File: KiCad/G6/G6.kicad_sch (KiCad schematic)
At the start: 7 parts, among them J2 Conn_02x20_Odd_Even_MountingP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, Q1 2N3904, U11 SN74HC74DRG4 (SOIC14)

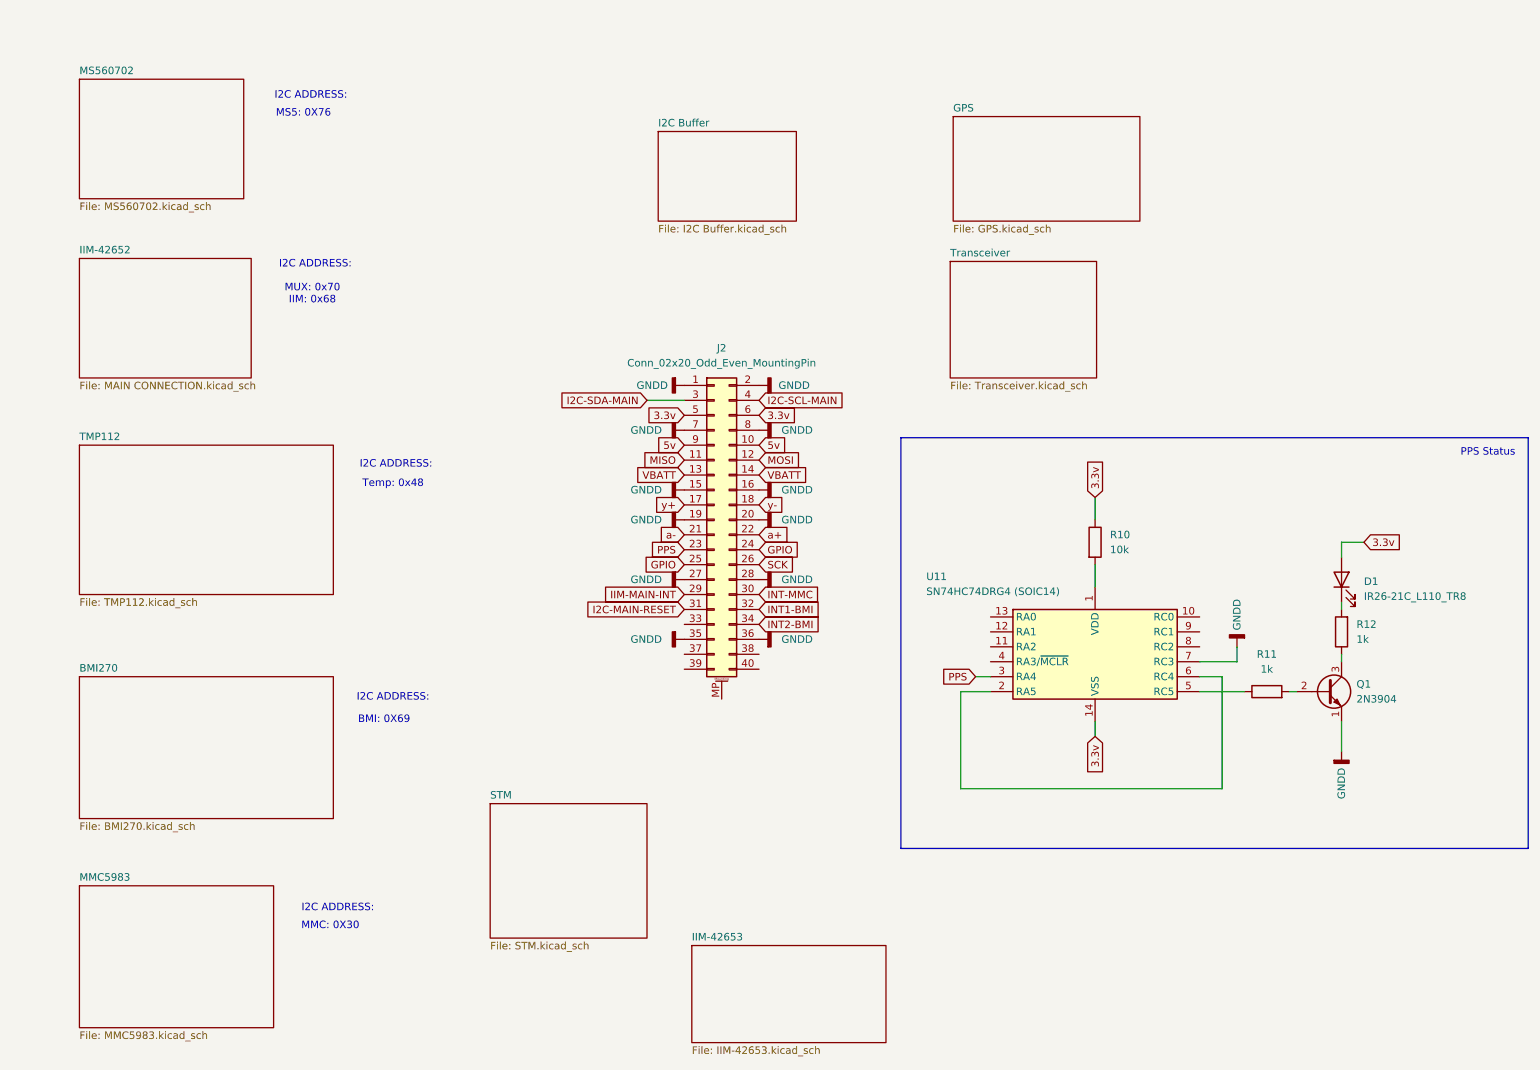
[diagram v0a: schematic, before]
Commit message: I think the schematics done uhhh idrk
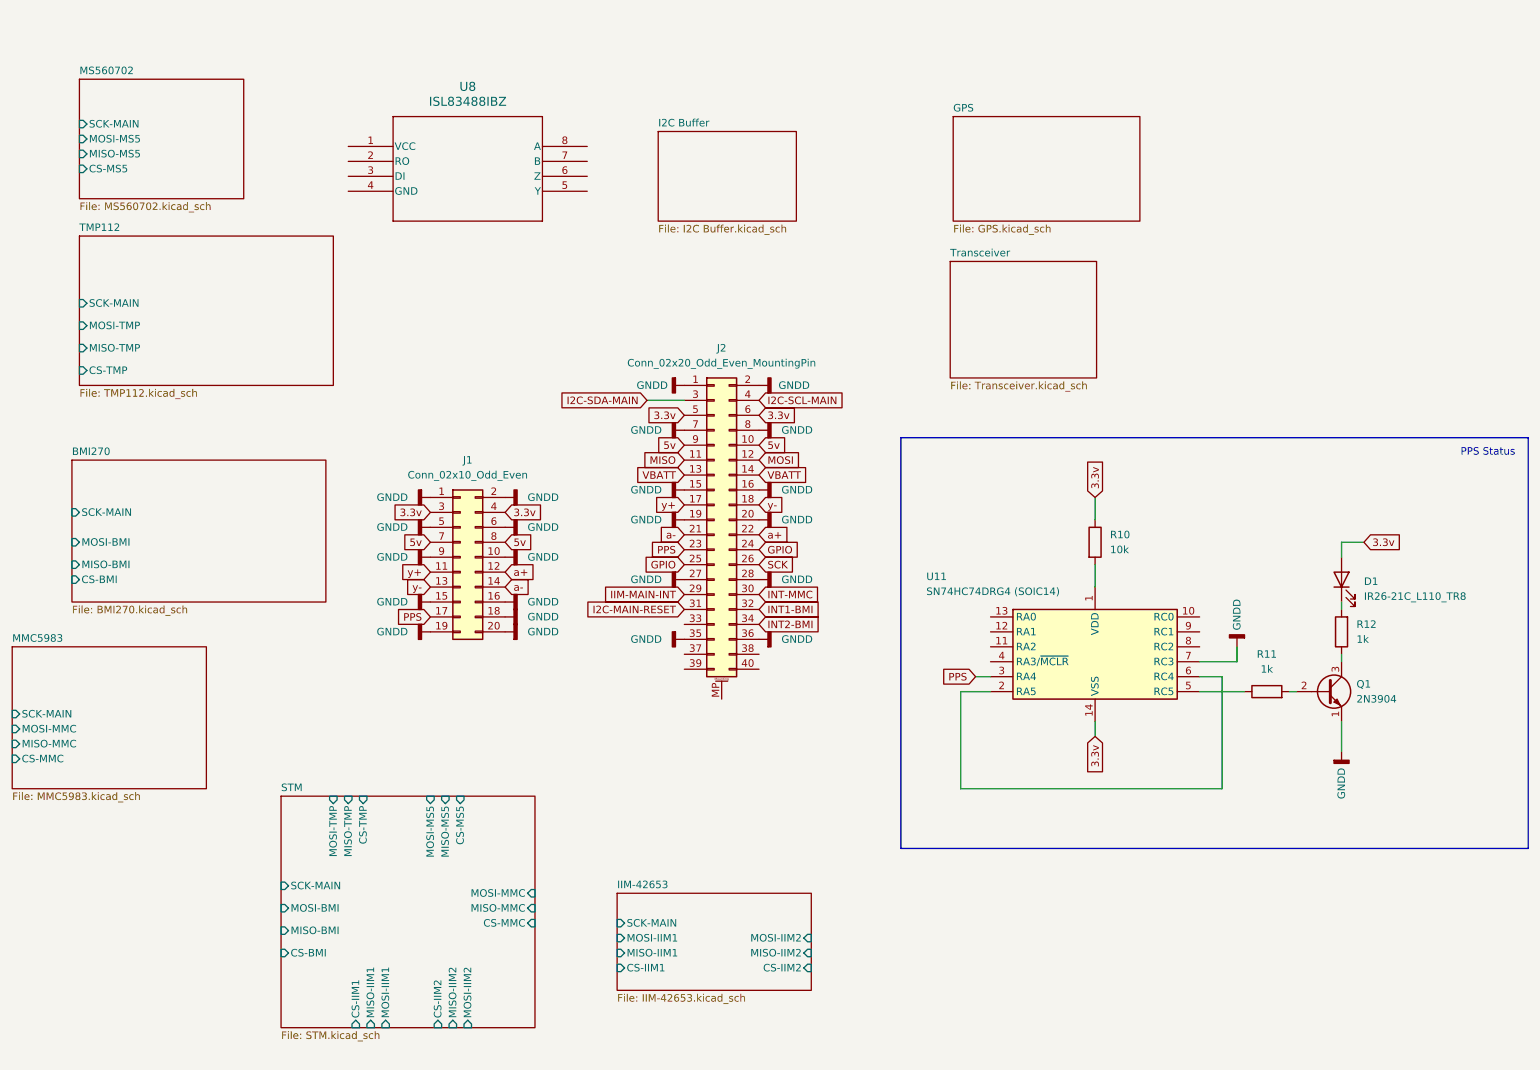
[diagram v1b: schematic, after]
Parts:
- added J1: Conn_02x10_Odd_Even, Connector_PinHeader_2.54mm:PinHeader_2x10_P2.54mm_Vertical, symbol Connector_Generic:Conn_02x10_Odd_Even
- added U8: ISL83488IBZ, CC0603KRXQRQBB104:SOIC8_4X5_INR, symbol ISL83488IBZ:ISL83488IBZ
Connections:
- net 3.3v: now also J1.3 (Pin_3), J1.4 (Pin_4)
- net 5v: now also J1.7 (Pin_7), J1.8 (Pin_8)
- net GNDD: now also J1.1 (Pin_1), J1.10 (Pin_10), J1.15 (Pin_15), J1.16 (Pin_16), J1.18 (Pin_18), J1.19 (Pin_19), J1.2 (Pin_2), J1.20 (Pin_20), J1.5 (Pin_5), J1.6 (Pin_6), J1.9 (Pin_9)
- net PPS: now also J1.17 (Pin_17)
- net a+: now also J1.12 (Pin_12)
- net a-: now also J1.14 (Pin_14)
- net y+: now also J1.11 (Pin_11)
- net y-: now also J1.13 (Pin_13)
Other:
- removed sheet IIM-42652
- sheet BMI270 ports: added CS-BMI, MISO-BMI, MOSI-BMI, SCK-MAIN; removed none
- sheet IIM-42653 ports: added CS-IIM1, CS-IIM2, MISO-IIM1, MISO-IIM2, MOSI-IIM1, MOSI-IIM2, SCK-MAIN; removed none
- sheet MMC5983 ports: added CS-MMC, MISO-MMC, MOSI-MMC, SCK-MAIN; removed none
- sheet MS560702 ports: added CS-MS5, MISO-MS5, MOSI-MS5, SCK-MAIN; removed none
- sheet STM ports: added CS-BMI, CS-IIM1, CS-IIM2, CS-MMC, CS-MS5, CS-TMP, MISO-BMI, MISO-IIM1, MISO-IIM2, MISO-MMC, MISO-MS5, MISO-TMP, MOSI-BMI, MOSI-IIM1, MOSI-IIM2, MOSI-MMC, MOSI-MS5, MOSI-TMP, SCK-MAIN; removed none
- sheet TMP112 ports: added CS-TMP, MISO-TMP, MOSI-TMP, SCK-MAIN; removed none
- note removed: "BMI: 0X69"
- note removed: "I2C ADDRESS:"
- note removed: "MMC: 0X30"
- note removed: "MS5: 0X76"
- note removed: "MUX: 0x70 IIM: 0x68"
- note removed: "Temp: 0x48"

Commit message: im sorry parsa :/
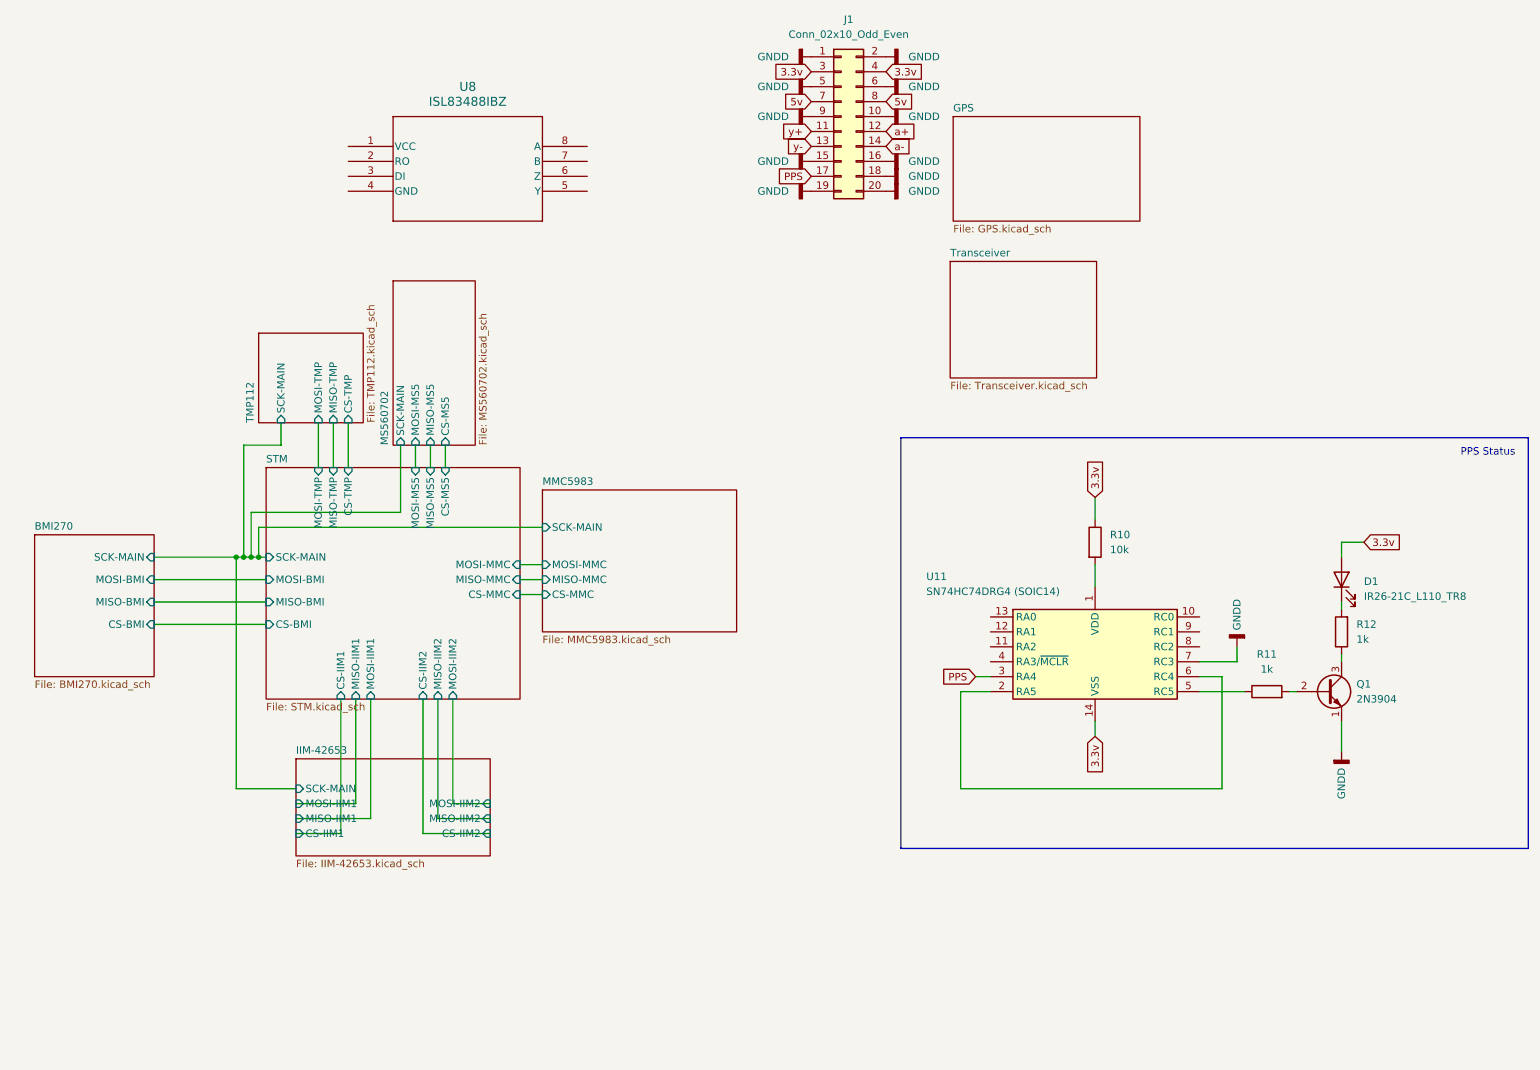
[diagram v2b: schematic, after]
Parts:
- removed J2: Conn_02x20_Odd_Even_MountingPin, Connector_PinHeader_2.54mm:PinHeader_2x20_P2.54mm_Vertical, symbol Connector_Generic_MountingPin:Conn_02x20_Odd_Even_MountingPin
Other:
- removed sheet I2C Buffer
- moved on the sheet: J1
